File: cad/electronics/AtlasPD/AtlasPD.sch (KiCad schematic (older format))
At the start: 1 part, among them U2 L78L05_SO8

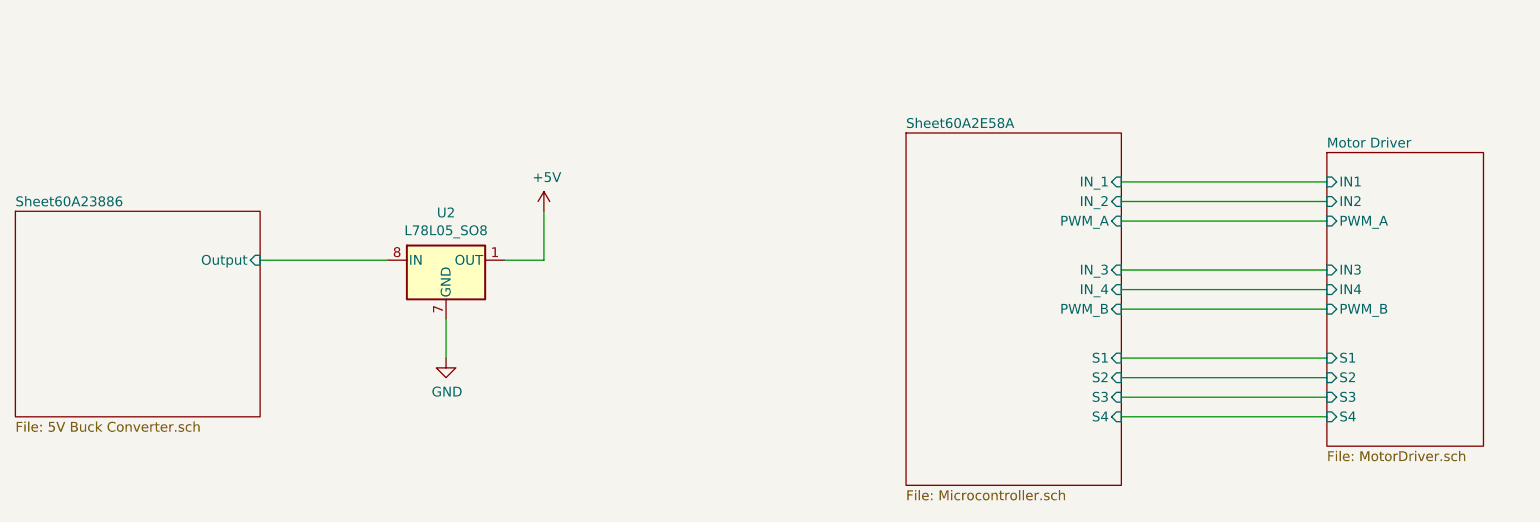
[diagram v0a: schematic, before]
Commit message: More Electronics design work
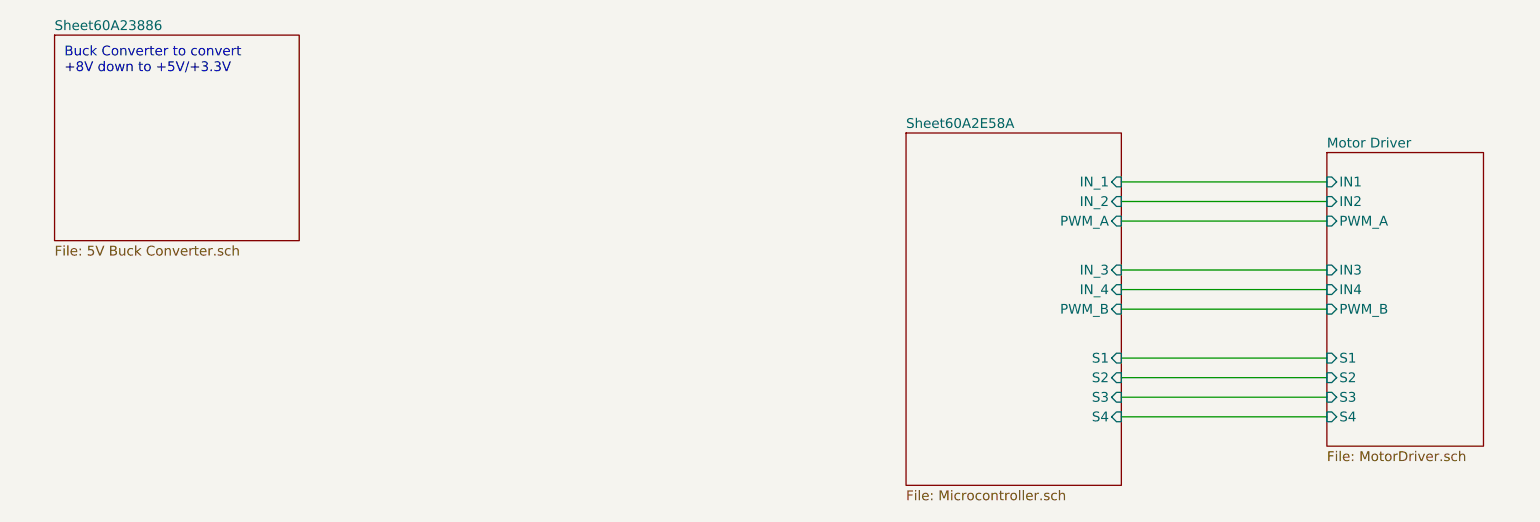
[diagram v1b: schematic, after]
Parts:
- removed U2: L78L05_SO8, Package_SO:SOIC-8_3.9x4.9mm_P1.27mm, symbol Regulator_Linear:L78L05_SO8
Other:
- note added: "Buck Converter to convert \n+8V down to +5V/+3.3V"
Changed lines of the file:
@@
 $EndDescr
-$Sheet
-S 1650 2300 1250 1050
-U 60A23887
-F0 "Sheet60A23886" 50
-F1 "5V Buck Converter.sch" 50
-F2 "Output" I R 2900 2550 50
-$EndSheet
 $Sheet
 S 6200 1900 1100 1800
@@
 Wire Wire Line
 	7300 3350 8350 3350
-$Comp
-L Regulator_Linear:L78L05_SO8 U2
-U 1 1 6141FB78
-P 3850 2550
-F 0 "U2" H 3850 2792 50  0000 C CNN
-F 1 "L78L05_SO8" H 3850 2701 50  0000 C CNN
-F 2 "Package_SO:SOIC-8_3.9x4.9mm_P1.27mm" H 3950 2750 50  0001 C CIN
-F 3 "http://www.st.com/content/ccc/resource/technical/document/datasheet/15/55/e5/aa/23/5b/43/fd/CD00000446.pdf/files/CD00000446.pdf/jcr:content/translations/en.CD00000446.pdf" H 4050 2550 50  0001 C CNN
-	1    3850 2550
-	1    0    0    -1
-$EndComp
-Wire Wire Line
-	2900 2550 3550 2550
-$Comp
-L power:+5V #PWR02
-U 1 1 61424002
-P 4350 2300
-F 0 "#PWR02" H 4350 2150 50  0001 C CNN
-F 1 "+5V" H 4365 2473 50  0000 C CNN
-F 2 "" H 4350 2300 50  0001 C CNN
-F 3 "" H 4350 2300 50  0001 C CNN
-	1    4350 2300
-	1    0    0    -1
-$EndComp
-Wire Wire Line
-	4350 2300 4350 2550
-Wire Wire Line
-	4350 2550 4150 2550
-$Comp
-L power:GND #PWR01
-U 1 1 614248BE
-P 3850 3050
-F 0 "#PWR01" H 3850 2800 50  0001 C CNN
-F 1 "GND" H 3855 2877 50  0000 C CNN
-F 2 "" H 3850 3050 50  0001 C CNN
-F 3 "" H 3850 3050 50  0001 C CNN
-	1    3850 3050
-	1    0    0    -1
-$EndComp
-Wire Wire Line
-	3850 2850 3850 3050
+$Sheet
+S 1850 1400 1250 1050
+U 60A23887
+F0 "Sheet60A23886" 50
+F1 "5V Buck Converter.sch" 50
+$EndSheet
+Text Notes 1900 1600 0    50   ~ 0
+Buck Converter to convert \n+8V down to +5V/+3.3V
 $EndSCHEMATC
